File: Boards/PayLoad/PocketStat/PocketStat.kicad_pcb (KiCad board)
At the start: 4 copper layers, 46 x 46 mm, 71 parts, among them J20 DX07S016JA1R1500, J3 MEM2061-01-188-00-A_REVA, J5 BM03B-SRSS-TBLFSN, Q1 BC857CMB_315, U1 HDC2080DMBR, U4 LPS22DFTR, U5 W25Q128JVSIQ TR, U6 BMP581, U8 ST1L05APU33R

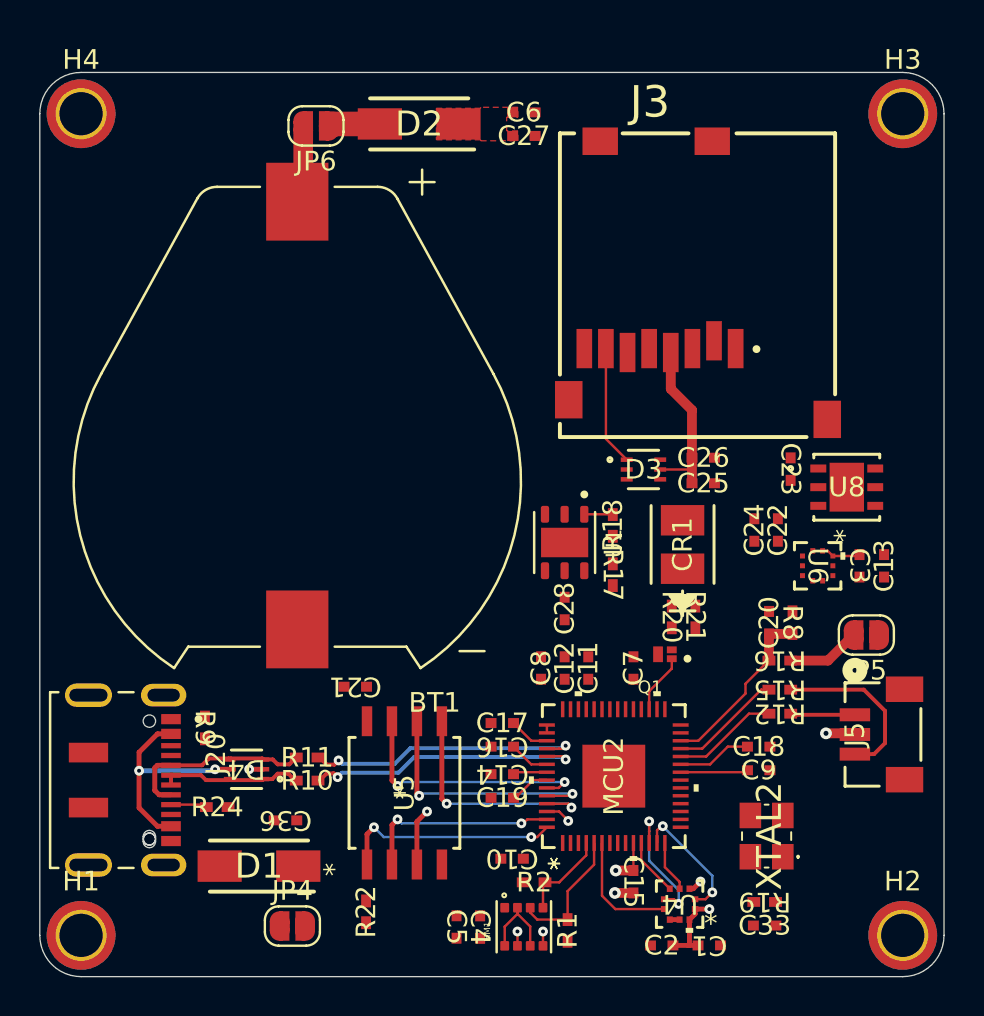
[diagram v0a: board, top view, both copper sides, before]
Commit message: PocketStat update
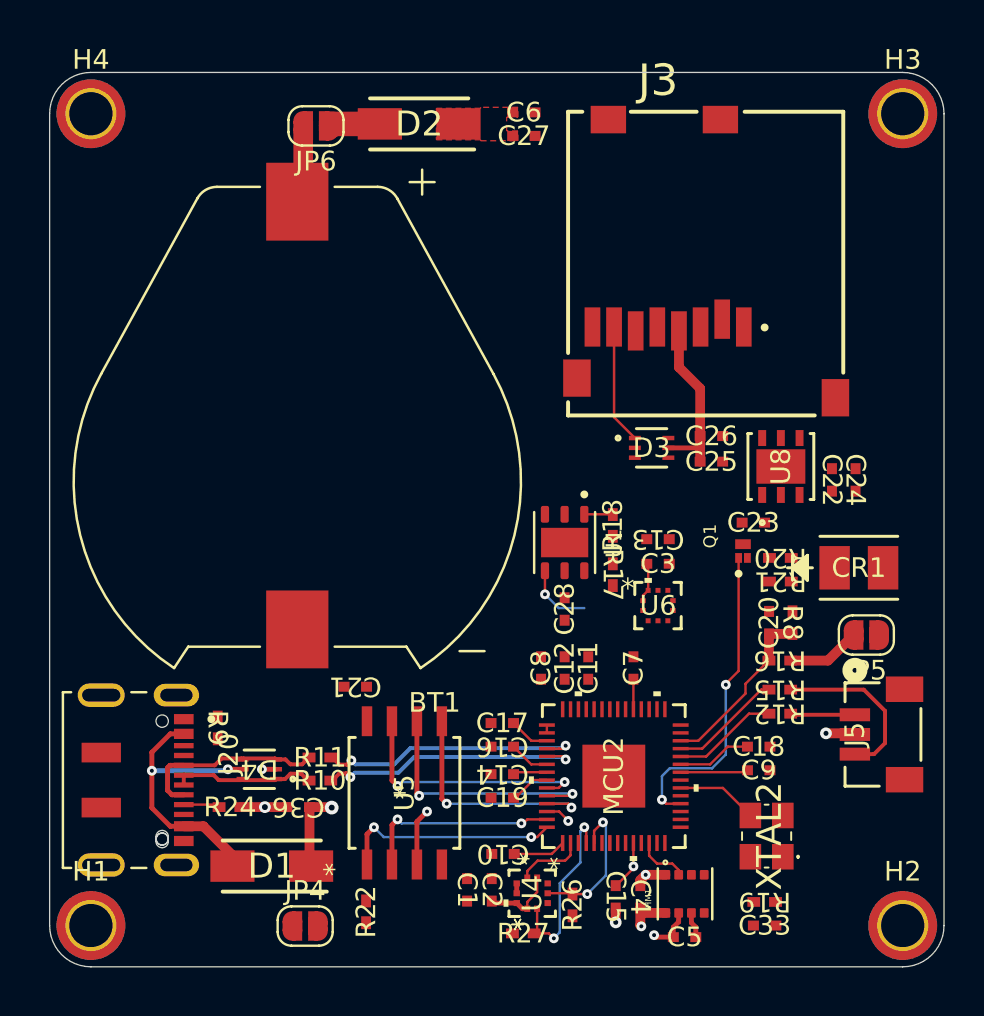
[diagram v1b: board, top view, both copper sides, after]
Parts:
- removed R1, R2: 2k, Resistor-0402:RES_0402
- added R26: 2k, Resistor-0402:RES_0402, F.Cu at (126.6, 96.9)
- added R27: 2k, Resistor-0402:RES_0402, F.Cu at (124.1, 98.3)
- moved C1 12.6 mm to (121.2, 96.1), turned to -90 degrees
- moved C5 11.6 mm to (132.3, 98.5), turned to 0 degrees
- moved C13 11.6 mm to (130.9, 78.2), turned to 180 degrees
- moved C3 10.3 mm to (130.9, 79.5), turned to 0 degrees
- moved C2 9.09 mm to (122.5, 96.1), turned to -90 degrees
- moved CR1 9.05 mm to (141.2, 79.7), turned to 0 degrees
- moved U6 8.37 mm to (130.9, 81.6), turned to 0 degrees
- moved HM1 8.37 mm to (132.3, 96.3)
- moved C4 8.29 mm to (130.1, 96.4)
- moved U4 7.52 mm to (124.5, 96.3), turned to 90 degrees
- moved Q1 6.59 mm to (135.3, 78.9), turned to 90 degrees
- moved R20 6.29 mm to (137.2, 79.2), turned to 180 degrees
- moved C24 5.75 mm to (141.0, 75.2), turned to -90 degrees
- moved R21 4.68 mm to (137.2, 80.4), turned to 180 degrees
- moved C22 3.75 mm to (139.8, 75.2), turned to -90 degrees
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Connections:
- HM1 pad 2: +3.3V -> /HUM ~{CS} SPI
- HM1 pad 3: /SDA1 I2C -> /MOSI1 SPI
- HM1 pad 4: /SCL1 I2C -> /SCK1 SPI
- HM1 pad 5: GND -> /MISO1 SPI
- MCU2 pad 12: /BAR1 ~{CS} SPI -> /HUM ~{CS} SPI
- MCU2 pad 15: /BAR2 RDY -> unconnected-(MCU2-GPIO12-Pad15)
- MCU2 pad 16: /BAR2 ~{CS} SPI -> unconnected-(MCU2-GPIO13-Pad16)
- MCU2 pad 18: unconnected-(MCU2-GPIO15-Pad18) -> /LED Status
- MCU2 pad 2: unconnected-(MCU2-GPIO0-Pad2) -> /BAR1 RDY
- MCU2 pad 31: /LED Status -> unconnected-(MCU2-GPIO20-Pad31)
- MCU2 pad 32: unconnected-(MCU2-GPIO21-Pad32) -> /BAR2 RDY
- MCU2 pad 35: /Humidity RDY -> unconnected-(MCU2-GPIO23-Pad35)
- MCU2 pad 38: unconnected-(MCU2-GPIO26_ADC0-Pad38) -> /Humidity RDY
- MCU2 pad 6: /BAR1 RDY -> unconnected-(MCU2-GPIO4-Pad6)
- U4 pad 2: /SCK1 SPI -> /SCL1 I2C
- U4 pad 4: /MOSI1 SPI -> /SDA1 I2C
- U4 pad 5: /MISO1 SPI -> GND
- U4 pad 6: /BAR1 ~{CS} SPI -> +3.3V
- U6 pad 2: /SCK1 SPI -> /SCL0 I2C
- U6 pad 4: /MOSI1 SPI -> /SDA0 I2C
- U6 pad 5: /MISO1 SPI -> GND
- U6 pad 6: /BAR2 ~{CS} SPI -> unconnected-(U6-CSB-Pad6)
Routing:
- net /LED Status: track 3.05 -> 16.2 mm, vias 0 -> 2
- net /BAR1 ~{CS} SPI: track 6.76 -> 0.00 mm, vias 2 -> 0
- net /SCK1 SPI: track 6.46 -> 0.00 mm, vias 2 -> 0
- net /SCL1 I2C: track 4.58 -> 9.56 mm, vias 0 -> 2
- net +6V: track 0.00 -> 4.17 mm, vias 0 -> 1
- net /Crystal: track 0.00 -> 4.13 mm
- net GND: track 5.94 -> 9.88 mm
- net +3.3V: track 29.2 -> 33.0 mm
- net VBUS: track 11.5 -> 15.2 mm
- net /Humidity RDY: track 0.00 -> 3.49 mm, vias 0 -> 1
- net /MISO1 SPI: track 2.92 -> 0.00 mm
- net /HUM ~{CS} SPI: track 0.00 -> 2.69 mm
- net /MOSI1 SPI: track 2.63 -> 0.00 mm
- net /BAR1 RDY: track 6.12 -> 3.50 mm
- net /D+: track 14.3 -> 13.7 mm
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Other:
- board size 46 x 46 mm -> 45.5 x 45.5 mm

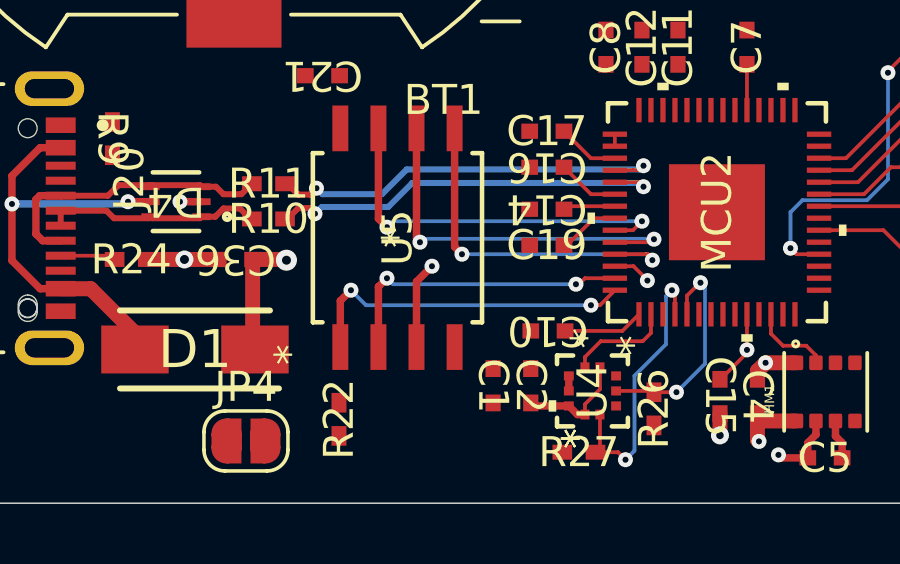
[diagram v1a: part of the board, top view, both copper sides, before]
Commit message: Pocket Stat Lib update
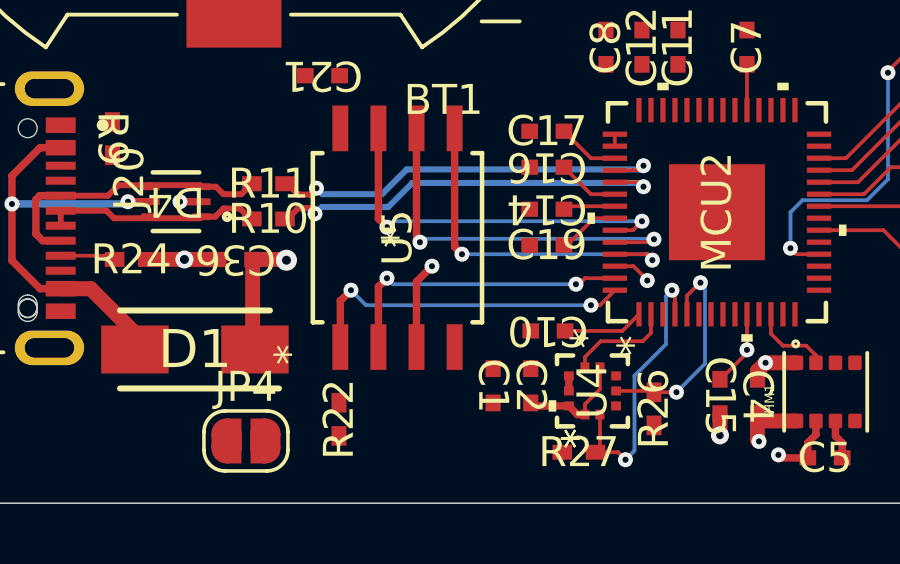
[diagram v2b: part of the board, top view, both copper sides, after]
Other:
- board text added: "TODO: 1- Fazer BOOM e atualizar excel de componentes 2- Routing crítico (Sinais Digitais) -> Fazer DRC no fim 3- Routing +3.3V -> Fazer DRC no fim 4- Routing +6V -> Fazer DRC no fim 5- Routing GND (Fazer ground planes) -> Fazer DRC no fim 6- Adicionar Test Points (GND, +3V3, +6V) 7- Fazer Silkscreen Bonito (Vai se ter de editar o Silkcreen de algumas footprints) (+ Assinar e Logo da PST) 8- Prepa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"
- board text removed: "TODO: 1- Routing crítico (Sinais Digitais) -> Fazer DRC no fim 2- Routing +3.3V -> Fazer DRC no fim 3- Routing +6V -> Fazer DRC no fim 4- Routing GND (Fazer ground planes) -> Fazer DRC no fim 5- Adicionar Test Points (GND, +3V3, +6V) 7- Fazer Silkscreen Bonito (Vai se ter de editar o Silkcreen de algumas footprints) (+ Assinar e Logo da PST) 8- Fazer BOOM e atualizar excel de componentes 9- Prepa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"
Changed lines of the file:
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@@
 			)
 		)
-		(fp_text user "${REFERENCE}"
-			(at 0 0 90)
+		(fp_text user "*"
+			(at -2.3114 -2.6162 90)
 			(unlocked yes)
 			(layer "F.Fab")
@@
 			)
 		)
-		(fp_text user "*"
-			(at -2.3114 -2.6162 90)
+		(fp_text user "${REFERENCE}"
+			(at 0 0 90)
 			(unlocked yes)
 			(layer "F.Fab")
@@
 		(layer "User.4")
 	)
-	(gr_text "TODO:\n1- Routing crítico (Sinais Digitais) -> Fazer DRC no fim\n2- Routing +3.3V -> Fazer DRC no fim\n3- Routing +6V  -> Fazer DRC no fim\n4- Routing GND (Fazer ground planes) -> Fazer DRC no fim\n5- Adicionar Test Points (GND, +3V3, +6V)\n7- Fazer Silkscreen Bonito\n(Vai se ter de editar o Silkcreen de algumas footprints)\n(+ Assinar e Logo da PST)\n8- Fazer BOOM e atualizar excel de componentes\n9- Preparar ficheiros de fabrico -> Tapeout\n---\nO Stackup é:\nTop Layer: Signal/PWR\nInner Layer 1: GND\nInner Layer 2: GND\nBottom Layer: Signal/PWR"
+	(gr_text "TODO:\n1- Fazer BOOM e atualizar excel de componentes\n2- Routing crítico (Sinais Digitais) -> Fazer DRC no fim\n3- Routing +3.3V -> Fazer DRC no fim\n4- Routing +6V  -> Fazer DRC no fim\n5- Routing GND (Fazer ground planes) -> Fazer DRC no fim\n6- Adicionar Test Points (GND, +3V3, +6V)\n7- Fazer Silkscreen Bonito\n(Vai se ter de editar o Silkcreen de algumas footprints)\n(+ Assinar e Logo da PST)\n8- Preparar ficheiros de fabrico -> Tapeout\n---\nO Stackup é:\nTop Layer: Signal/PWR\nInner Layer 1: GND\nInner Layer 2: GND\nBottom Layer: Signal/PWR"
 		(at 99.4 142.45 0)
 		(layer "User.1")
@@
 		(net 6)
 	)
-	(segment
-		(start 113.221499 94.796501)
-		(end 113.3 94.875002)
-		(width 0.5)
-		(layer "F.Cu")
-		(net 6)
-	)
 	(via
 		(at 114.349999 91.9)
@@
 	)
 	(segment
-		(start 125.2 81.05)
-		(end 125.9 81.75)
+		(start 125.9 81.75)
+		(end 127.2 81.75)
 		(width 0.125)
 		(layer "B.Cu")
@@
 	)
 	(segment
-		(start 125.9 81.75)
-		(end 127.2 81.75)
+		(start 125.2 81.05)
+		(end 125.9 81.75)
 		(width 0.125)
 		(layer "B.Cu")
@@
 	)
 	(segment
-		(start 126.381009 92.578145)
+		(start 126.381009 92.573519)
 		(end 126.381009 92.56231)
 		(width 0.125)
@@
 	)
 	(segment
-		(start 118.685 92.615)
-		(end 119.2 92.1)
-		(width 0.25)
+		(start 126.377296 92.577232)
+		(end 126.381009 92.573519)
+		(width 0.125)
 		(layer "F.Cu")
 		(net 52)
 	)
 	(segment
-		(start 126.381009 92.56231)
-		(end 125.918698 92.099999)
-		(width 0.125)
+		(start 118.685 92.615)
+		(end 119.2 92.1)
+		(width 0.25)
 		(layer "F.Cu")
 		(net 52)
@@
 		(net 52)
 	)
+	(segment
+		(start 126.381009 92.56231)
+		(end 125.918698 92.099999)
+		(width 0.125)
+		(layer "F.Cu")
+		(net 52)
+	)
 	(via
 		(at 119.2 92.1)
@@
 	)
 	(via
-		(at 126.381009 92.578145)
+		(at 126.377296 92.577232)
 		(size 0.5)
 		(drill 0.2)
@@
 	)
 	(segment
-		(start 126.4 91.7)
-		(end 125.2964 91.7)
+		(start 126.546312 91.846312)
+		(end 126.4 91.7)
 		(width 0.125)
 		(layer "F.Cu")
@@
 	)
 	(segment
-		(start 126.546312 91.846312)
-		(end 126.4 91.7)
+		(start 126.4 91.7)
+		(end 125.2964 91.7)
 		(width 0.125)
 		(layer "F.Cu")
@@
 	)
 	(segment
-		(start 126.348372 91.7)
-		(end 120.2 91.7)
+		(start 126.546312 91.89794)
+		(end 126.348372 91.7)
 		(width 0.125)
 		(layer "B.Cu")
@@
 	)
 	(segment
-		(start 126.546312 91.89794)
-		(end 126.348372 91.7)
+		(start 126.348372 91.7)
+		(end 120.2 91.7)
 		(width 0.125)
 		(layer "B.Cu")

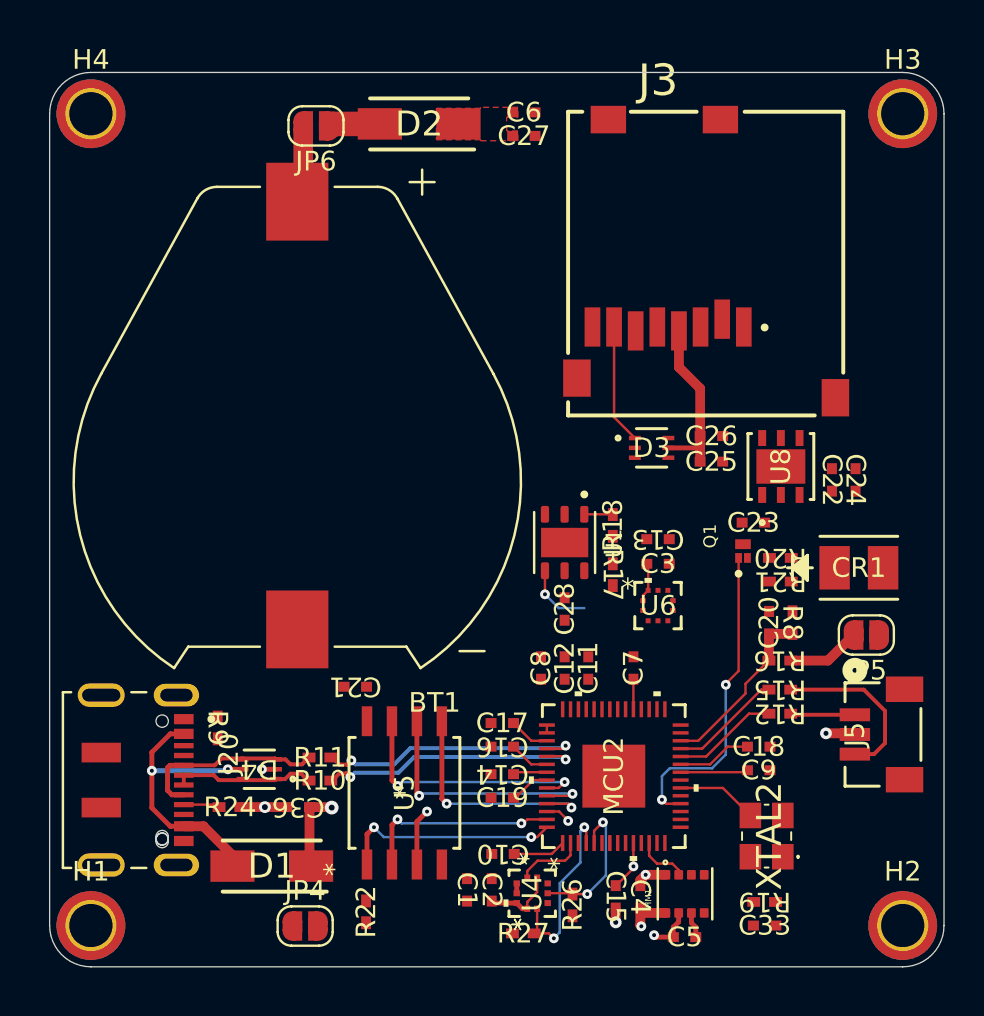
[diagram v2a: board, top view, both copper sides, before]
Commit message: pocketstat power update
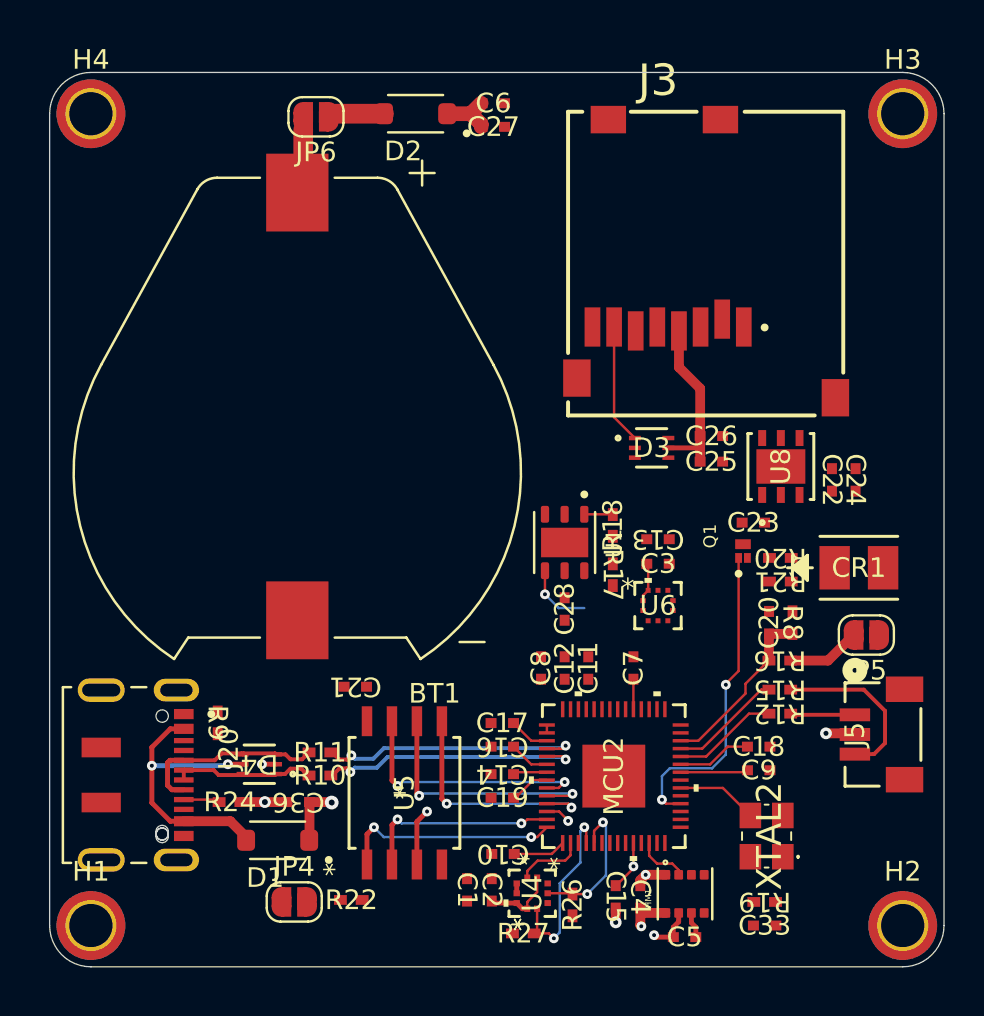
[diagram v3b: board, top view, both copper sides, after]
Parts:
- D1, D2: value RSX301L-30DDTE25 -> PMEG2010ER; footprint Diode-Schottky_RSX301L:DIOM5026X220N -> Diode-Schottky_PMEG2010ER:SODFL3517X110N
- moved C27 1.62 mm to (122.6, 57.3)
- moved C6 1.62 mm to (122.6, 56.1)
- moved D1 1.35 mm to (111.6, 93.6)
- moved JP4 1.35 mm to (112.4, 96.7)
- moved R22 0.96 mm to (115.3, 96.6), turned to 0 degrees
- moved D2 0.55 mm to (118.6, 56.6)
- moved JP6 0.46 mm to (113.6, 56.8)
- moved BT1 0.46 mm to (112.6, 71.5)
- moved R10 0.26 mm to (113.7, 90.3)
- moved C36 0.26 mm to (112.6, 91.6)
- moved D4 0.26 mm to (110.7, 89.7)
- moved J20 0.26 mm to (105.7, 90.2)
- moved R11 0.26 mm to (113.7, 89.1)
- moved R24 0.26 mm to (109.2, 91.6)
- moved R9 0.26 mm to (108.5, 87.6)
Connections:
- C22 pad 2: +6V -> +5V
- C24 pad 2: +6V -> +5V
- C27 pad 1: +6V -> +5V
- C36 pad 1: +6V -> +5V
- C6 pad 1: +6V -> +5V
- CR1 pad 2: +6V -> +5V
- JP6 pad 1: Net-(D2-A) -> Net-(JP6-A)
- U8 pad 3: +6V -> +5V
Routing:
- net +5V: track 0.00 -> 5.93 mm, vias 0 -> 1
- net +6V: track 4.06 -> 0.00 mm, vias 1 -> 0
- net Net-(JP6-A): track 0.00 -> 2.88 mm
- net Net-(D2-A): track 2.52 -> 0.00 mm
- removed copper zone on F.Cu, net +6V
